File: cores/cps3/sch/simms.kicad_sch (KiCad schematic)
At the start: 0 parts

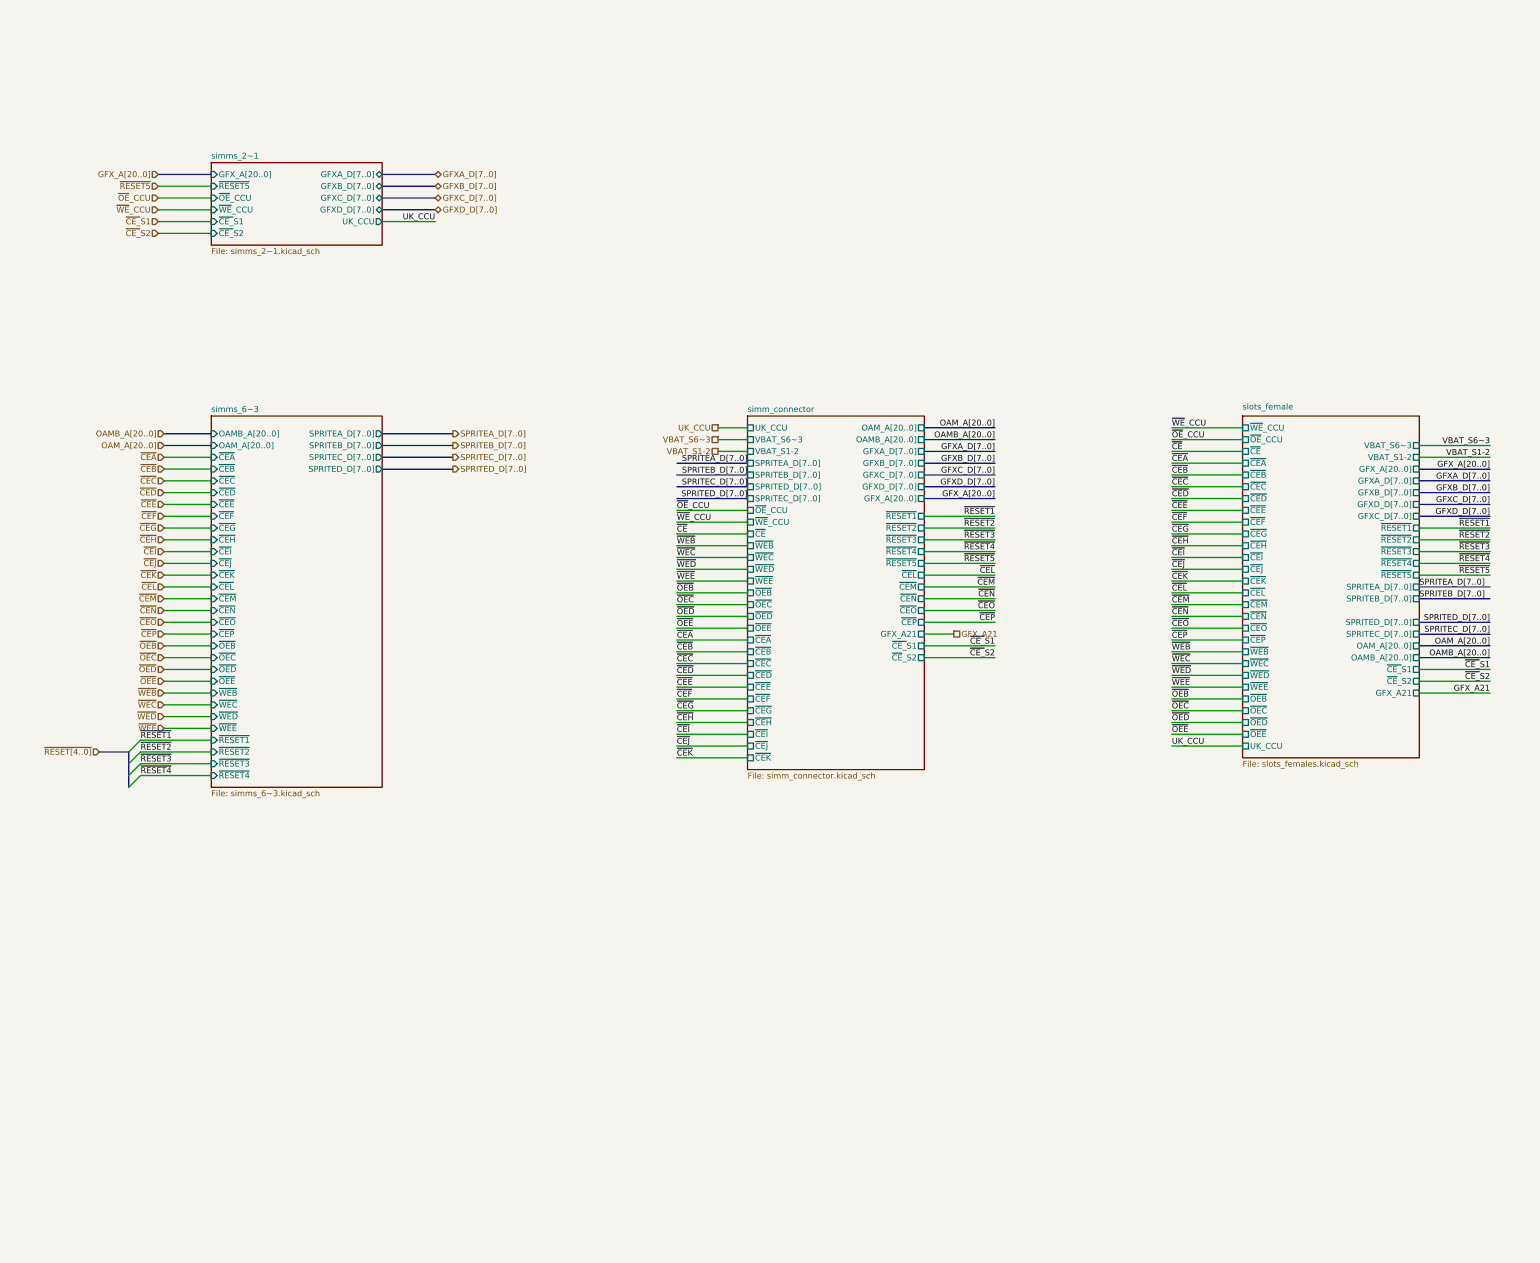
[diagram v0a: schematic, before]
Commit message: wip_cassette_sh2
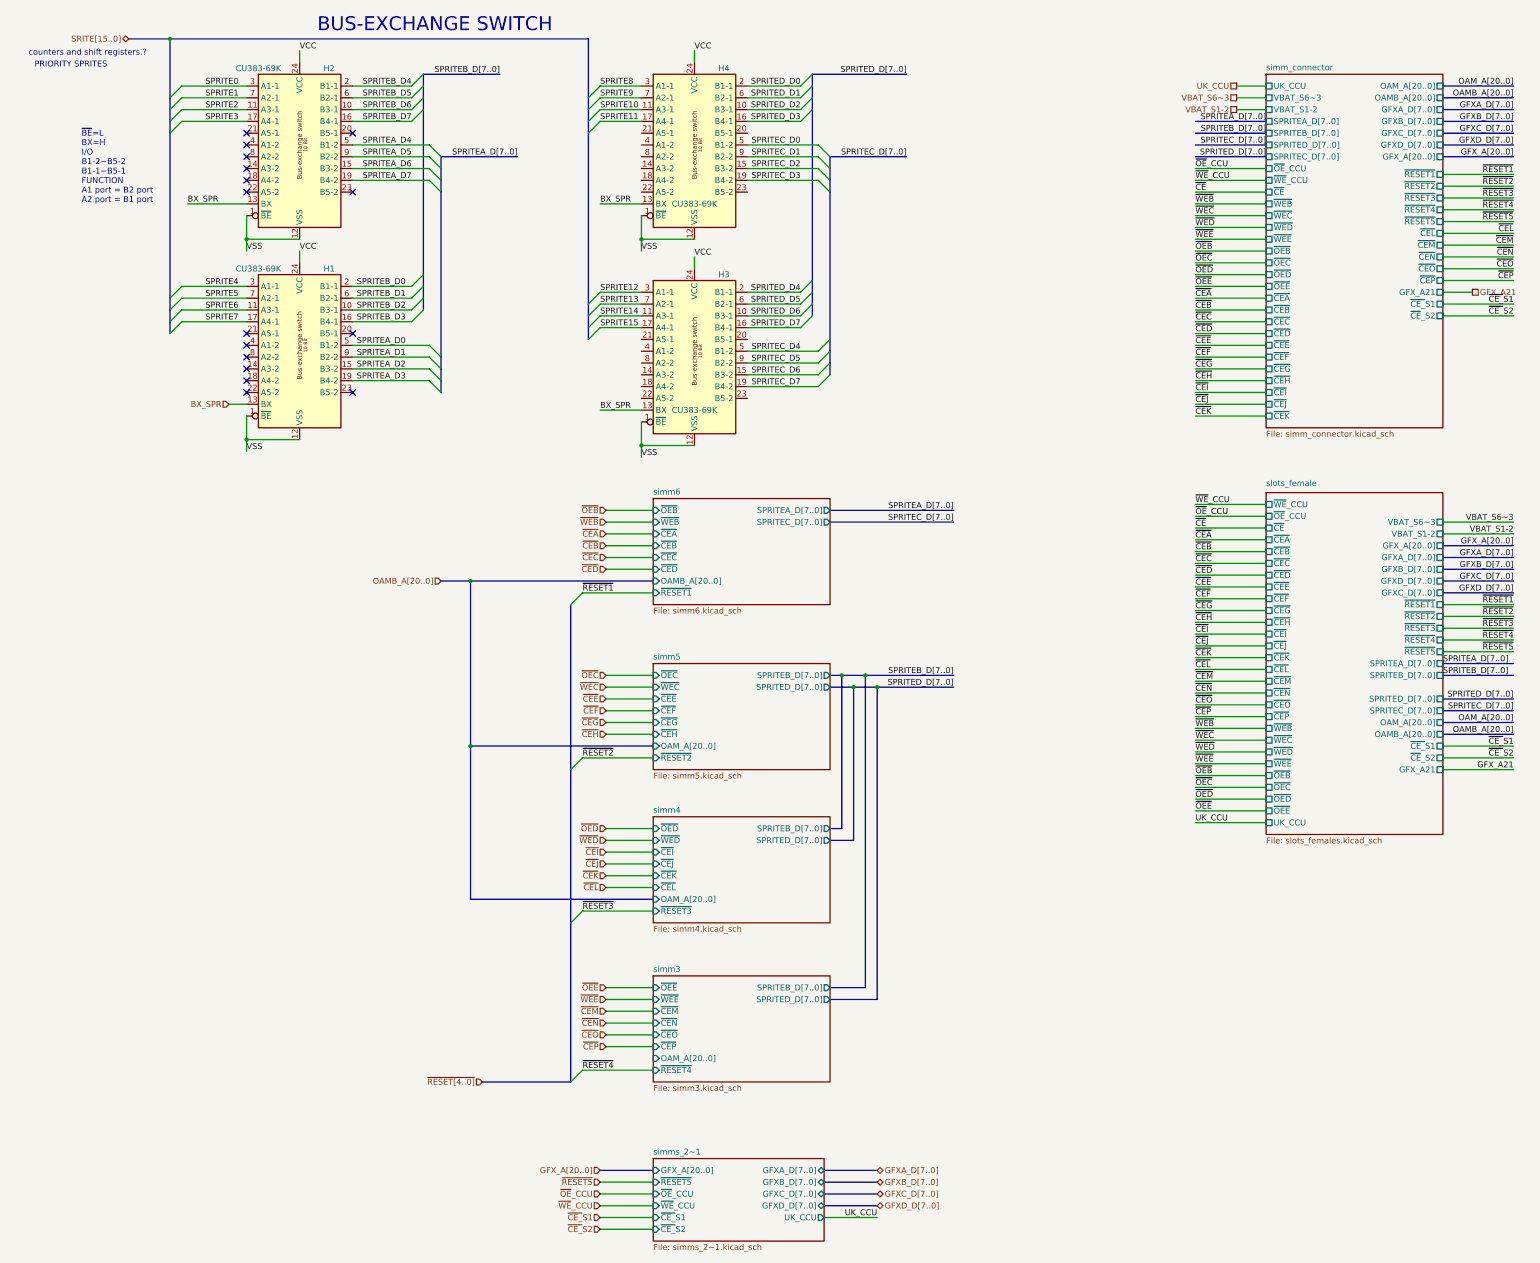
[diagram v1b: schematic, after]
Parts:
- added H1, H2, H3, H4: CU383-69K, symbol arcade:CU383-69K
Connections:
- new net BX_SPR: H1.13 (BX), H2.13 (BX), H3.13 (BX), H4.13 (BX)
- new net SPRITE0: H2.3 (A1-1)
- new net SPRITE1: H2.7 (A2-1)
- new net SPRITE10: H4.11 (A3-1)
- new net SPRITE11: H4.17 (A4-1)
- new net SPRITE12: H3.3 (A1-1)
- new net SPRITE13: H3.7 (A2-1)
- new net SPRITE14: H3.11 (A3-1)
- new net SPRITE15: H3.17 (A4-1)
- new net SPRITE2: H2.11 (A3-1)
- new net SPRITE3: H2.17 (A4-1)
- new net SPRITE4: H1.3 (A1-1)
- new net SPRITE5: H1.7 (A2-1)
- new net SPRITE6: H1.11 (A3-1)
- new net SPRITE7: H1.17 (A4-1)
- new net SPRITE8: H4.3 (A1-1)
- new net SPRITE9: H4.7 (A2-1)
- new net SPRITEA_D0: H1.5 (B1-2)
- new net SPRITEA_D1: H1.9 (B2-2)
- new net SPRITEA_D2: H1.15 (B3-2)
- new net SPRITEA_D3: H1.19 (B4-2)
- new net SPRITEA_D4: H2.5 (B1-2)
- new net SPRITEA_D5: H2.9 (B2-2)
- new net SPRITEA_D6: H2.15 (B3-2)
- new net SPRITEA_D7: H2.19 (B4-2)
- new net SPRITEB_D0: H1.2 (B1-1)
- new net SPRITEB_D1: H1.6 (B2-1)
- new net SPRITEB_D2: H1.10 (B3-1)
- new net SPRITEB_D3: H1.16 (B4-1)
- new net SPRITEB_D4: H2.2 (B1-1)
- new net SPRITEB_D5: H2.6 (B2-1)
- new net SPRITEB_D6: H2.10 (B3-1)
- new net SPRITEB_D7: H2.16 (B4-1)
- new net SPRITEC_D0: H4.5 (B1-2)
- new net SPRITEC_D1: H4.9 (B2-2)
- new net SPRITEC_D2: H4.15 (B3-2)
- new net SPRITEC_D3: H4.19 (B4-2)
- new net SPRITEC_D4: H3.5 (B1-2)
- new net SPRITEC_D5: H3.9 (B2-2)
- new net SPRITEC_D6: H3.15 (B3-2)
- new net SPRITEC_D7: H3.19 (B4-2)
- new net SPRITED_D0: H4.2 (B1-1)
- new net SPRITED_D1: H4.6 (B2-1)
- new net SPRITED_D2: H4.10 (B3-1)
- new net SPRITED_D3: H4.16 (B4-1)
- new net SPRITED_D4: H3.2 (B1-1)
- new net SPRITED_D5: H3.6 (B2-1)
- new net SPRITED_D6: H3.10 (B3-1)
- new net SPRITED_D7: H3.16 (B4-1)
- new net VCC: H1.24 (VCC), H2.24 (VCC), H3.24 (VCC), H4.24 (VCC)
- new net VSS: H1.1 (~{BE}), H1.12 (VSS), H2.1 (~{BE}), H2.12 (VSS), H3.1 (~{BE}), H3.12 (VSS), H4.1 (~{BE}), H4.12 (VSS)
- no-connect marks 0 -> 16
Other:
- sheet simms_6~3 renamed simm3
- added sheet simm4 (simm4.kicad_sch)
- added sheet simm5 (simm5.kicad_sch)
- added sheet simm6 (simm6.kicad_sch)
- sheet simm3: file simms_6~3.kicad_sch -> simm3.kicad_sch
- sheet simm3 ports: added none; removed OAMB_A[20..0], SPRITEA_D[7..0], SPRITEC_D[7..0], ~{CEA}, ~{CEB}, ~{CEC}, ~{CED}, ~{CEE}, ~{CEF}, ~{CEG}, ~{CEH}, ~{CEI}, ~{CEJ}, ~{CEK}, ~{CEL}, ~{OEB}, ~{OEC}, ~{OED}, ~{RESET1}, ~{RESET2}, ~{RESET3}, ~{WEB}, ~{WEC}, ~{WED}
- note added: "BUS-EXCHANGE SWITCH"
- note added: "PRIORITY SPRITES"
- note added: "counters and shift registers.?"
- note added: "~{BE}=L BX=H I/O B1-2−B5-2 B1-1−B5-1 FUNCTION A1 port = B2 port A2 port = B1 port"
